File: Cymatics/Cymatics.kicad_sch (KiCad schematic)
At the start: 68 parts, among them IC1 LMV358IDR, IC2 MAX7403CSA+, IC3 LMV358IDR, IC4 LMV358IDR, IC5 MAX7403CSA+, J1 Screw_Terminal_01x03, J10 Screw_Terminal_01x04, J11 Screw_Terminal_01x05, J12 Screw_Terminal_01x02, J13 Screw_Terminal_01x02, J15 Screw_Terminal_01x02, J16 Screw_Terminal_01x03, J17 Screw_Terminal_01x02, J18 Screw_Terminal_01x06, J2 Screw_Terminal_01x02, J3 Screw_Terminal_01x03, J4 Screw_Terminal_01x03, J5 Screw_Terminal_01x02, J6 Conn_01x16_Socket, J7 Conn_01x12_Socket, J8 Screw_Terminal_01x04, J9 Screw_Terminal_01x02, U1 SN74AHCT125DR, U2 MAX7480ESA+

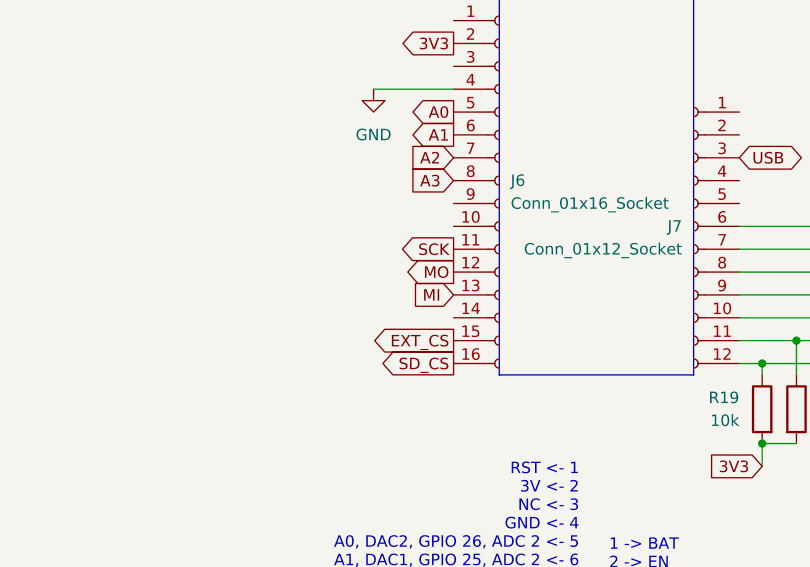
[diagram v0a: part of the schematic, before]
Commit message: resolved all DRC errors
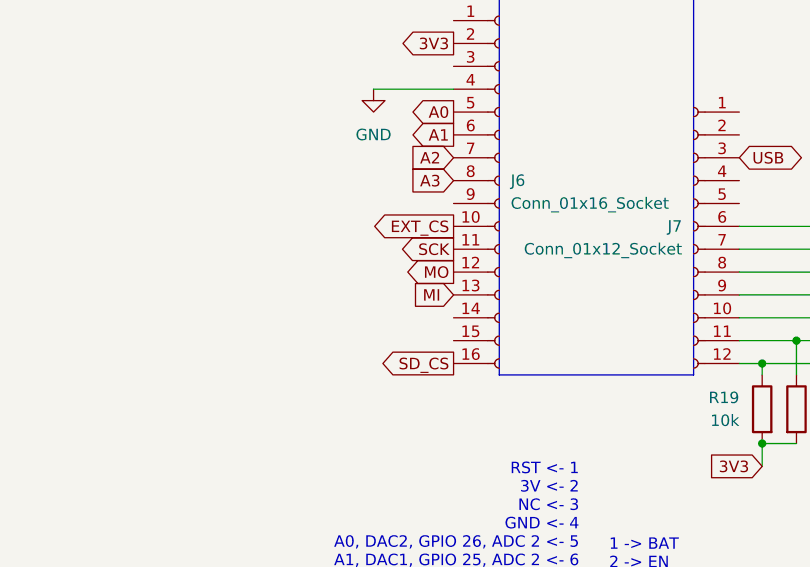
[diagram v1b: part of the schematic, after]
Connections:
- net EXT_CS: now also J6.10 (Pin_10); no longer J6.15 (Pin_15)
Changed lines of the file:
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@@
-		)
-	)
-	(global_label "EXT_CS"
-		(shape output)
-		(at 147.32 226.06 180)
-		(fields_autoplaced yes)
-		(effects
-			(font
-				(size 1.27 1.27)
-			)
-			(justify right)
-		)
-		(property "Intersheetrefs" "${INTERSHEET_REFS}"
-			(at 137.5616 226.06 0)
-			(effects
-				(font
-					(size 1.27 1.27)
-				)
-				(justify right)
-				(hide yes)
-			)
 		)
 	)
@@
 				(hide yes)
 			)
+		)
+	)
+	(global_label "EXT_CS"
+		(shape output)
+		(at 147.32 213.36 180)
+		(fields_autoplaced yes)
+		(effects
+			(font
+				(size 1.27 1.27)
+			)
+			(justify right)
+		)
+		(property "Intersheetrefs" "${INTERSHEET_REFS}"
+			(at 137.5616 213.36 0)
+			(effects
+				(font
+					(size 1.27 1.27)
+				)
+				(justify right)
+				(hide yes)
+			)
